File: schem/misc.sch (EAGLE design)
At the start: 4 parts, among them IC1 74HC377N, IC2 74HC244N, IC3 74HC377N, IC4 74HC244N

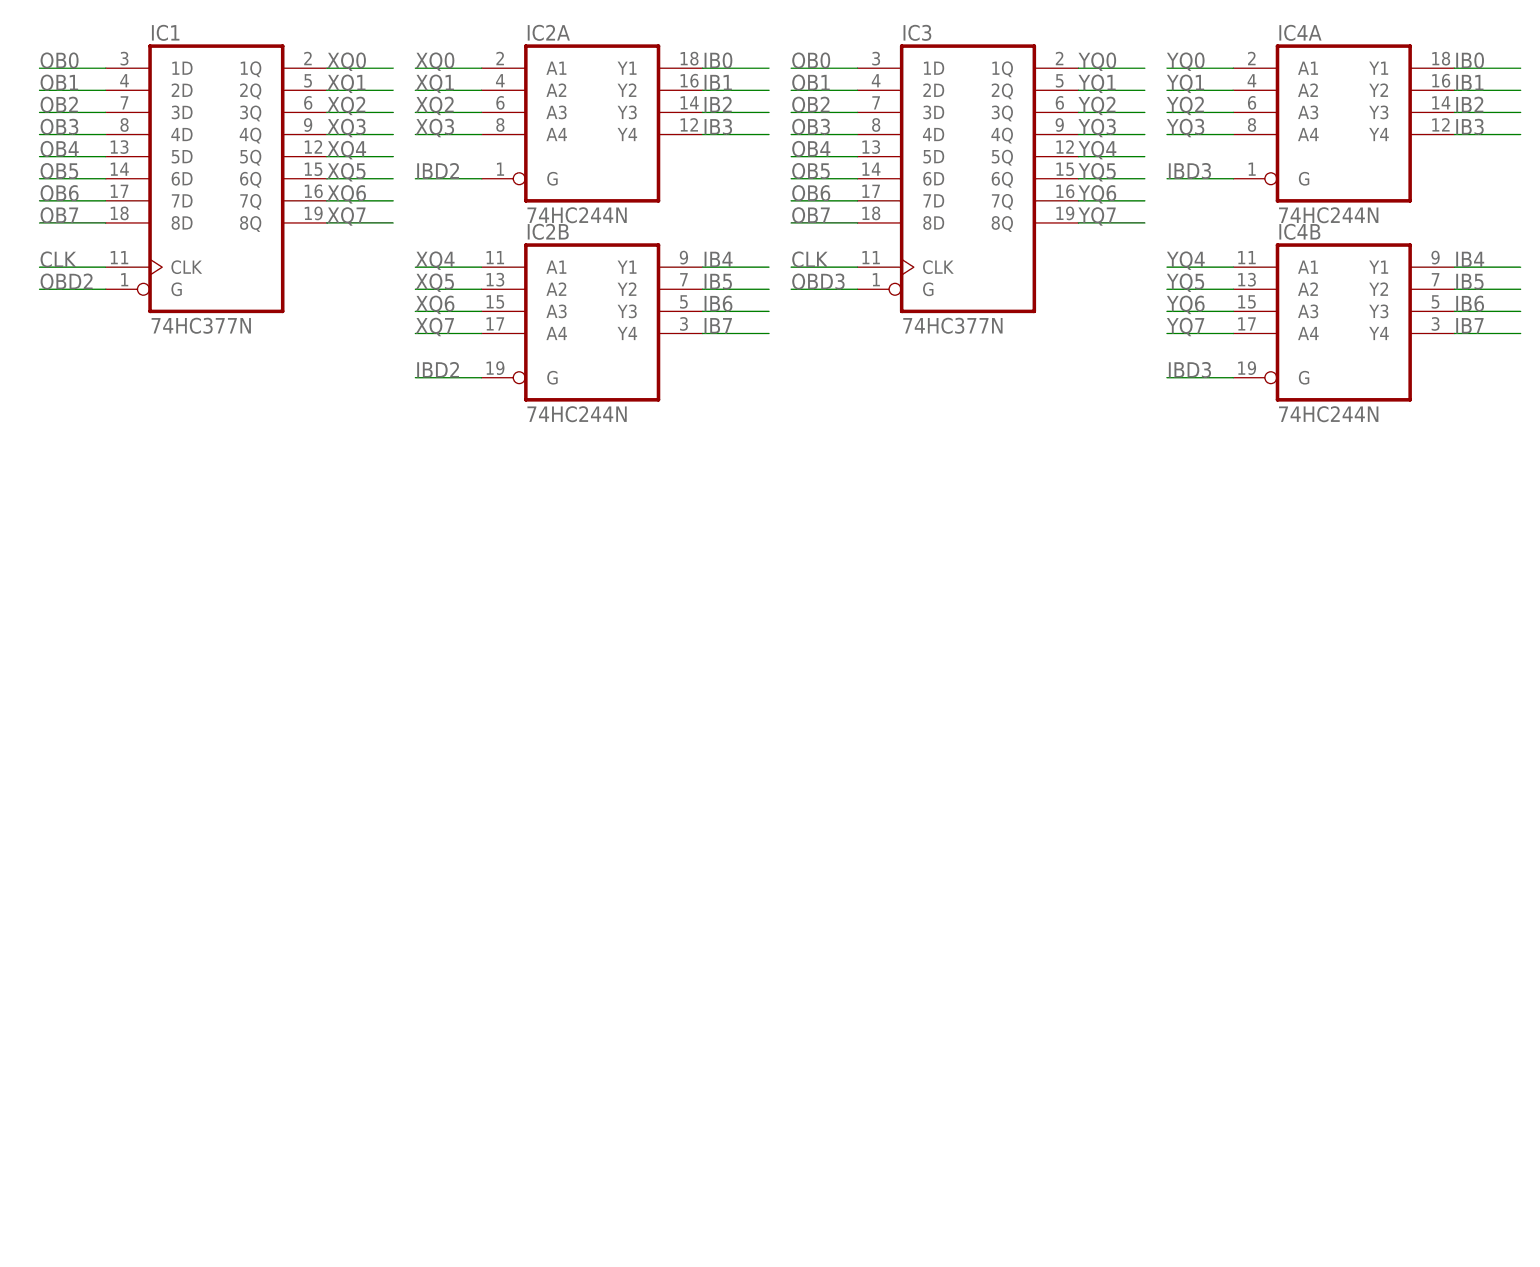
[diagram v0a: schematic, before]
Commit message: progress
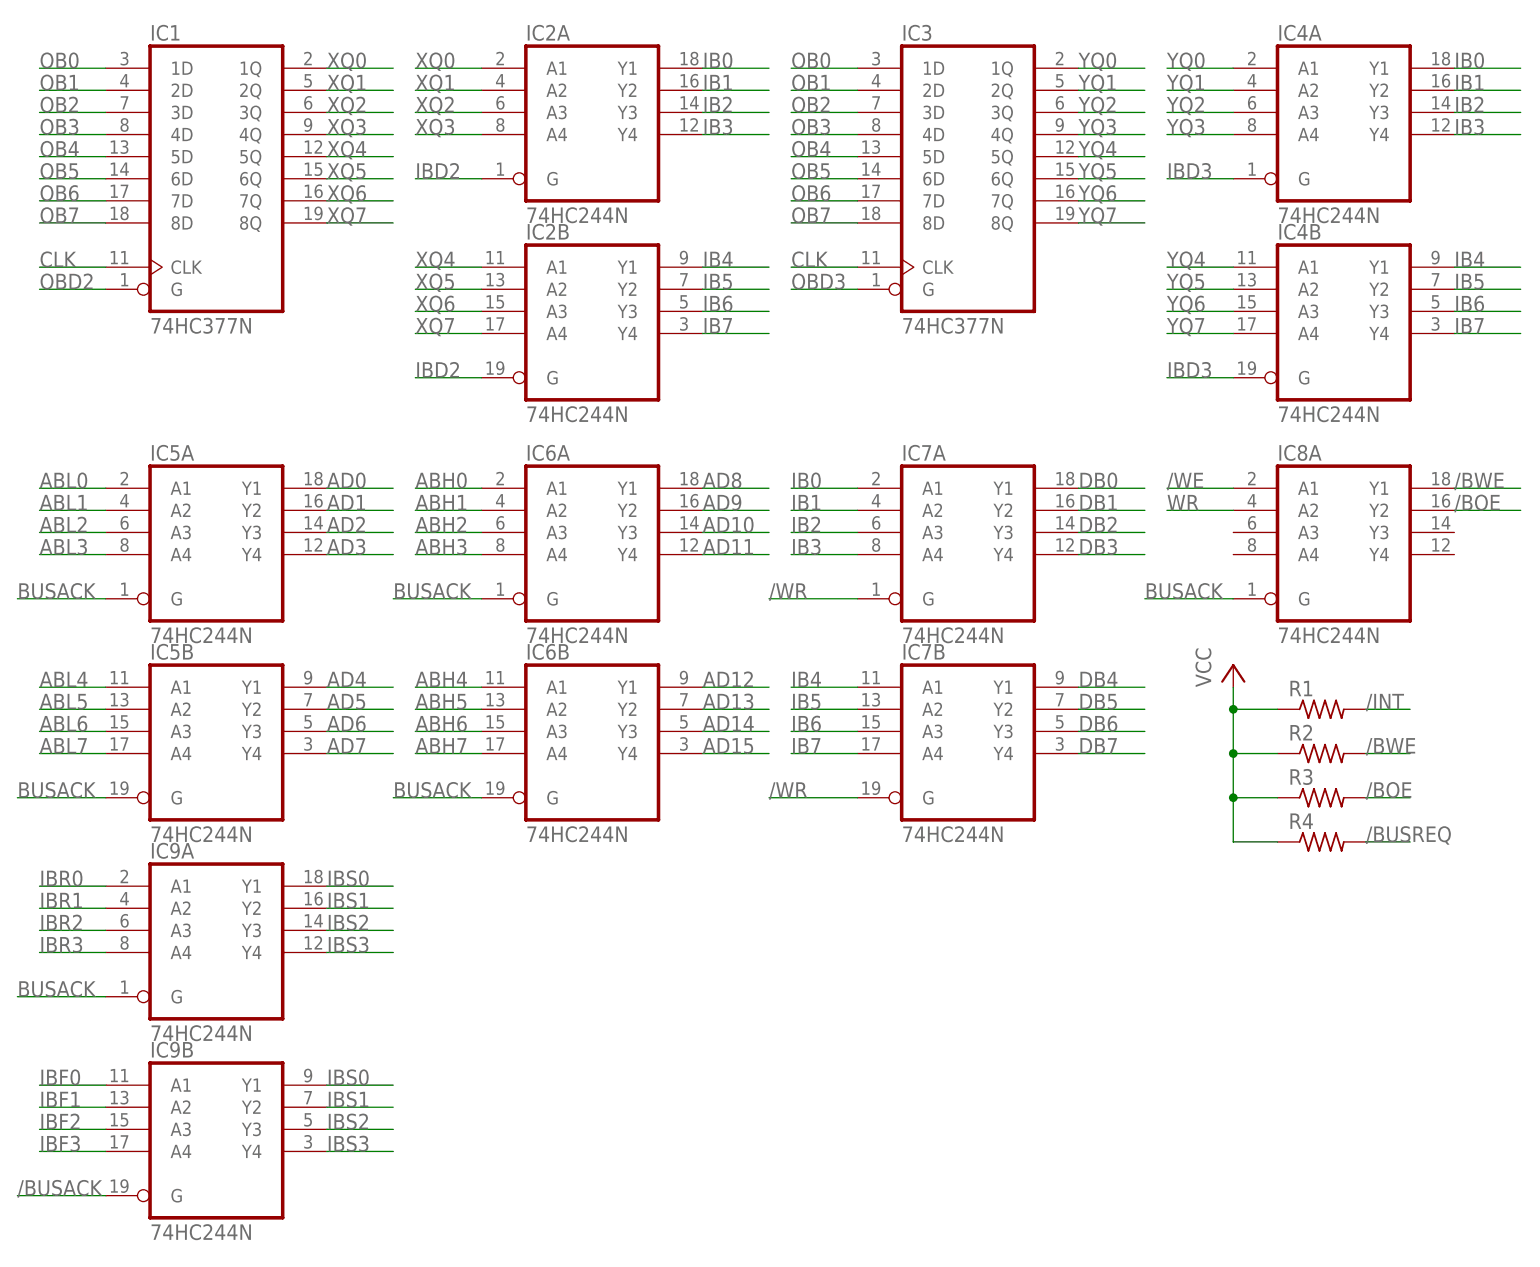
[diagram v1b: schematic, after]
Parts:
- added IC5, IC6, IC7, IC8, IC9: 74HC244N, 74xx-eu:74HC244N
- added R1, R2, R3, R4: (no value), rcl:R-US_0207/10
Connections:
- new net /BOE: IC8A.Y2, R3.2
- new net /BUSACK: IC9B.G
- new net /BUSREQ: R4.2
- new net /BWE: IC8A.Y1, R2.2
- new net /INT: R1.2
- new net /WE: IC8A.A1
- new net /WR: IC7A.G, IC7B.G
- new net ABH0: IC6A.A1
- new net ABH1: IC6A.A2
- new net ABH2: IC6A.A3
- new net ABH3: IC6A.A4
- new net ABH4: IC6B.A1
- new net ABH5: IC6B.A2
- new net ABH6: IC6B.A3
- new net ABH7: IC6B.A4
- new net ABL0: IC5A.A1
- new net ABL1: IC5A.A2
- new net ABL2: IC5A.A3
- new net ABL3: IC5A.A4
- new net ABL4: IC5B.A1
- new net ABL5: IC5B.A2
- new net ABL6: IC5B.A3
- new net ABL7: IC5B.A4
- new net AD0: IC5A.Y1
- new net AD1: IC5A.Y2
- new net AD10: IC6A.Y3
- new net AD11: IC6A.Y4
- new net AD12: IC6B.Y1
- new net AD13: IC6B.Y2
- new net AD14: IC6B.Y3
- new net AD15: IC6B.Y4
- new net AD2: IC5A.Y3
- new net AD3: IC5A.Y4
- new net AD4: IC5B.Y1
- new net AD5: IC5B.Y2
- new net AD6: IC5B.Y3
- new net AD7: IC5B.Y4
- new net AD8: IC6A.Y1
- new net AD9: IC6A.Y2
- new net BUSACK: IC5A.G, IC5B.G, IC6A.G, IC6B.G, IC8A.G, IC9A.G
- new net DB0: IC7A.Y1
- new net DB1: IC7A.Y2
- new net DB2: IC7A.Y3
- new net DB3: IC7A.Y4
- new net DB4: IC7B.Y1
- new net DB5: IC7B.Y2
- new net DB6: IC7B.Y3
- new net DB7: IC7B.Y4
- new net IBF0: IC9B.A1
- new net IBF1: IC9B.A2
- new net IBF2: IC9B.A3
- new net IBF3: IC9B.A4
- new net IBR0: IC9A.A1
- new net IBR1: IC9A.A2
- new net IBR2: IC9A.A3
- new net IBR3: IC9A.A4
- new net IBS0: IC9A.Y1, IC9B.Y1
- new net IBS1: IC9A.Y2, IC9B.Y2
- new net IBS2: IC9A.Y3, IC9B.Y3
- new net IBS3: IC9A.Y4, IC9B.Y4
- new net VCC: R1.1, R2.1, R3.1, R4.1
- new net WR: IC8A.A2
- net IB0: now also IC7A.A1
- net IB1: now also IC7A.A2
- net IB2: now also IC7A.A3
- net IB3: now also IC7A.A4
- net IB4: now also IC7B.A1
- net IB5: now also IC7B.A2
- net IB6: now also IC7B.A3
- net IB7: now also IC7B.A4
